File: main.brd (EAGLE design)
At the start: 120 x 120 mm, 578 parts, among them CN1 50 PIN 0.5MM, CN2 10067847-001RLF, CN3 632723300011, CN4 FF0881SA1, CN5 15PIN 0.5MM, CN6 31 PIN FPC, Q1 2N7002, Q2 FDN302P, Q3 2N7002, Q5 SI7489DP, SW2 TACT, SW3 TACT, SW4 TACT, SW5 TACT, SW7 TACT, SW8 SLIDE SPDT, U1 GMAX0505-DV, U10 TPS70950, U11 FT601Q, U12 CBTU02043, U13 MAX25300B, U14 ESP32, U15 MAX25300B, U16 INA180, U17 AP62301, U18 AP62301, U19 SCHMITT, U2 XC7Z014S-1CLG484C, U20 MAX25300B, U21 NOT, U22 MAX25300B, U23 SN74LVC1G3, U24 NAND, U25 EMC1812T, U26 BIPOLAR HALL, U27 LM2663, U28 ADS7867, U29 LM2663, U3 IS43TR16128CL-125KBLI, U30 LM2731X, U31 USBLC6-2SC6, U32 MAX1735, U33 MP2148, U34 TPS22917, U35 AP62301, U36 TLV61046A, U37 W25Q128JV, U38 TPS70918, U39 AP62301, U4 AP63300WU-7, U5 STM32L431RBT, U6 USB ESD, U7 ACT2861QI301-T, U8 TPS70918, U9 STUSB4500

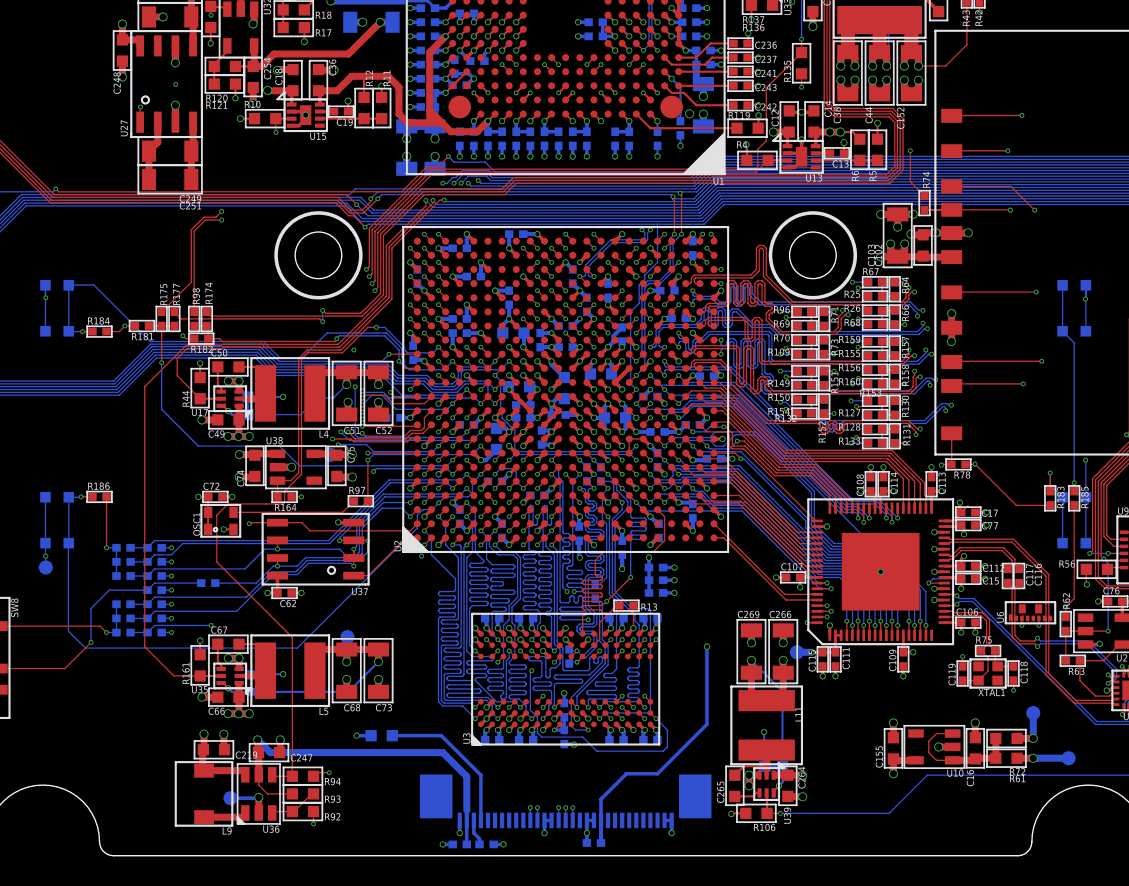
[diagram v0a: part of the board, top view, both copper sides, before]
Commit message: Correct FPGA footprint routed. A lot of work to length match, optimise and review
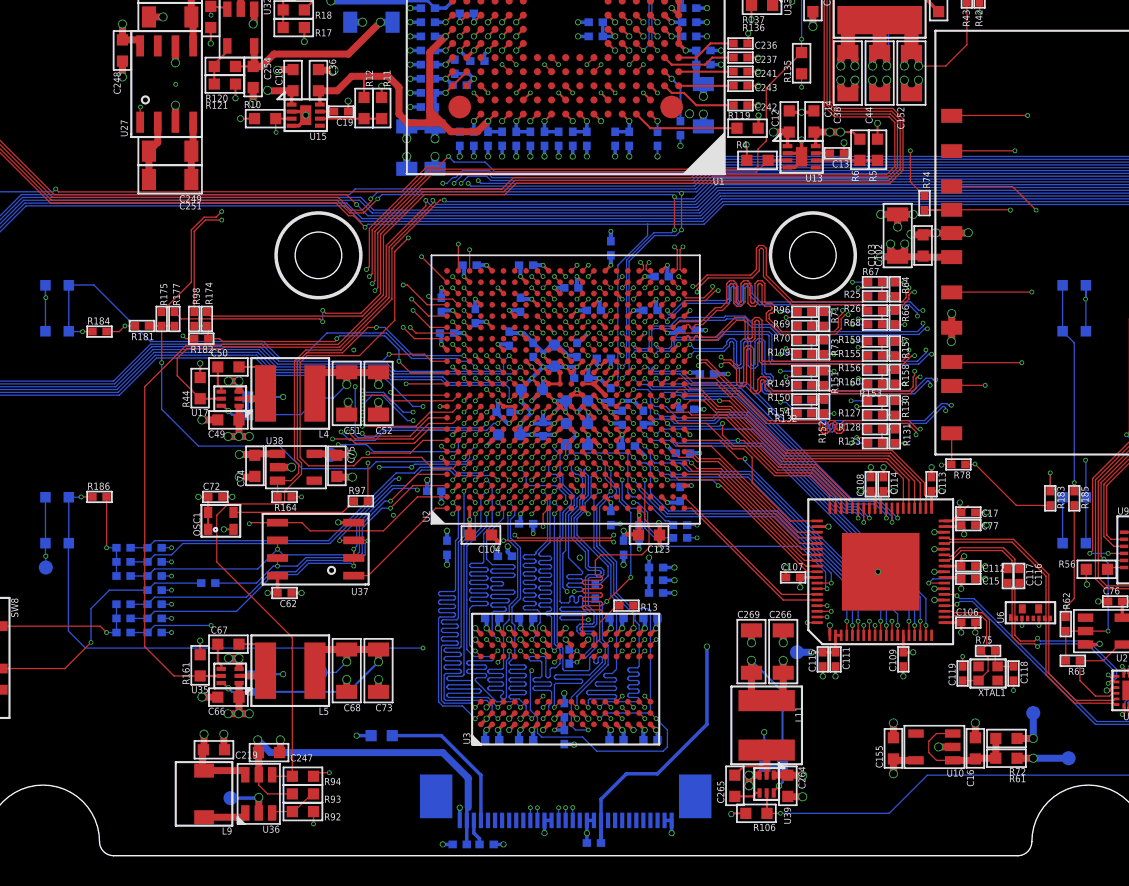
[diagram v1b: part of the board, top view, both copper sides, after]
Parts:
- removed C124, C126: 0.1uF 10V, c_0402:0402
- C104, C123: value 0.1uF 10V -> 47uF 6.3V; device c_0402:0402 -> c_0603:0603
- U2: device ICs:FBGA484 -> ICs:CLG484
- moved C131 17.3 mm to (6.80, -19.0)
- moved C123 16.9 mm to (5.90, -37.3), flipped to the top, turned to 180 degrees
- moved C132 13.9 mm to (0.80, -24.2), turned to 90 degrees
- moved C133 12.1 mm to (0.40, -19.8), turned to 0 degrees
- moved C104 8.83 mm to (-6.00, -37.3), flipped to the top
- moved C127 8.27 mm to (2.00, -21.4), turned to 180 degrees
- moved C138 7.57 mm to (-3.20, -21.0), turned to 270 degrees
- moved R1 7.52 mm to (8.10, -36.6), turned to 0 degrees
- moved R2 7.18 mm to (8.10, -37.5), turned to 180 degrees
- moved C128 6.53 mm to (10.0, -25.9)
- moved C86 5.71 mm to (0.80, -30.9), turned to 180 degrees
- moved C120 4.50 mm to (4.00, -29.0), turned to 90 degrees
- moved C186 4.36 mm to (-9.30, -34.2), turned to 180 degrees
- moved C83 4.21 mm to (-2.40, -27.0), turned to 0 degrees
- moved C122 4.20 mm to (3.20, -27.4), turned to 270 degrees
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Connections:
- removed net N$19: U2.M20
- removed net N$31: U2.M19
- net DDR_D0: now also U2.E1; no longer U2.E3
- net DDR_D2: now also U2.G2; no longer U2.G1
- net DDR_D4: now also U2.L2; no longer U2.L1
- net DDR_D6: now also U2.L1; no longer U2.L2
- net DDR_D8: now also U2.G1; no longer U2.G2
- net DDR_D9: now also U2.E3; no longer U2.E1
- net FT_BE0: now also U2.V4; no longer U2.U4
- net FT_BE1: now also U2.U6; no longer U2.Y5
- net FT_BE3: now also U2.U5; no longer U2.V5
- net FT_D0: now also U2.AA12; no longer U2.AB12
- net FT_D1: now also U2.AB12; no longer U2.AA12
- net FT_D10: now also U2.W10; no longer U2.V10
- net FT_D11: now also U2.AB10; no longer U2.Y10
- net FT_D12: now also U2.Y10; no longer U2.AB10
- net FT_D24: now also U2.U4; no longer U2.V4
- net FT_D29: now also U2.T6; no longer U2.R7
- net FT_D3: now also U2.AA11; no longer U2.AB11
- net FT_D30: now also U2.R7; no longer U2.T6
- net FT_D4: now also U2.AB11; no longer U2.AA11
- net FT_D6: now also U2.V12; no longer U2.U12
- net FT_D7: now also U2.U12; no longer U2.V12
- net FT_GPIO0: now also U2.W8; no longer U2.V8
- net FT_GPIO1: now also U2.V10; no longer U2.W10
- net FT_NRESET: now also U2.V8; no longer U2.Y8
- net FT_NSIWU: now also U2.Y5; no longer U2.U6
- net FT_NTXE: now also U2.V5; no longer U2.U5
- net FT_NWAKEUP: now also U2.Y8; no longer U2.W8
- net GND: no longer C124.1, C126.1
- net PWR_ANA_1V8: no longer C104.2
- net PWR_DDR3_1V35: now also C104.2, C123.2
- net PWR_SEN_0V7_EN: now also U2.A9; no longer U2.B10
- net PWR_SEN_N1V3A_EN: now also U2.B10; no longer U2.A9
- net PWR_SYS_1V8: no longer C123.2, C124.2, C126.2
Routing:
- net BTN_TOPLEFT: track 56.6 -> 108.3 mm
- net BTN_BTMLEFT: track 52.6 -> 103.9 mm, vias 3 -> 2
- net PSS_SD_D0: track 75.0 -> 47.5 mm
- net PSS_SD_D1: track 74.9 -> 48.4 mm
- net PSS_SD_CLK: track 74.7 -> 57.2 mm
- net SEN_B_D12_N: track 35.1 -> 22.5 mm
- net SEN_B_D12_P: track 35.1 -> 22.8 mm
- net N$42: track 1.41 -> 13.1 mm, vias 1 -> 2
- net N$7: track 1.41 -> 12.8 mm
- net PSS_SD_D3: track 74.8 -> 63.9 mm
- net PSS_SD_CMD: track 75.3 -> 65.3 mm
- net PSS_NRST: track 143.9 -> 153.5 mm
- net DDR_A10: track 25.0 -> 15.8 mm
- net PWR_SYS_3V3: track 177.0 -> 168.8 mm
- net BTN_BTMRIGHT: track 43.4 -> 51.3 mm, vias 2 -> 3
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
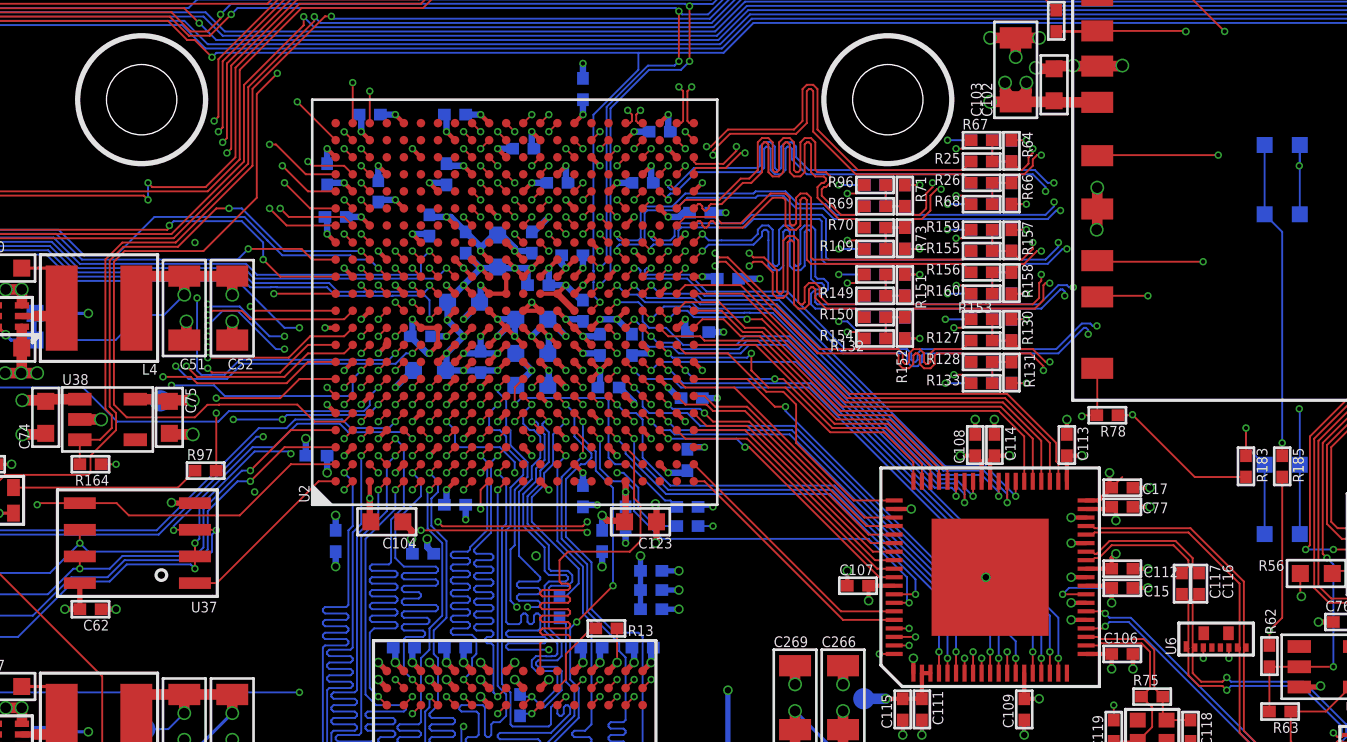
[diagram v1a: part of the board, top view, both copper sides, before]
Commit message: Passes DRC
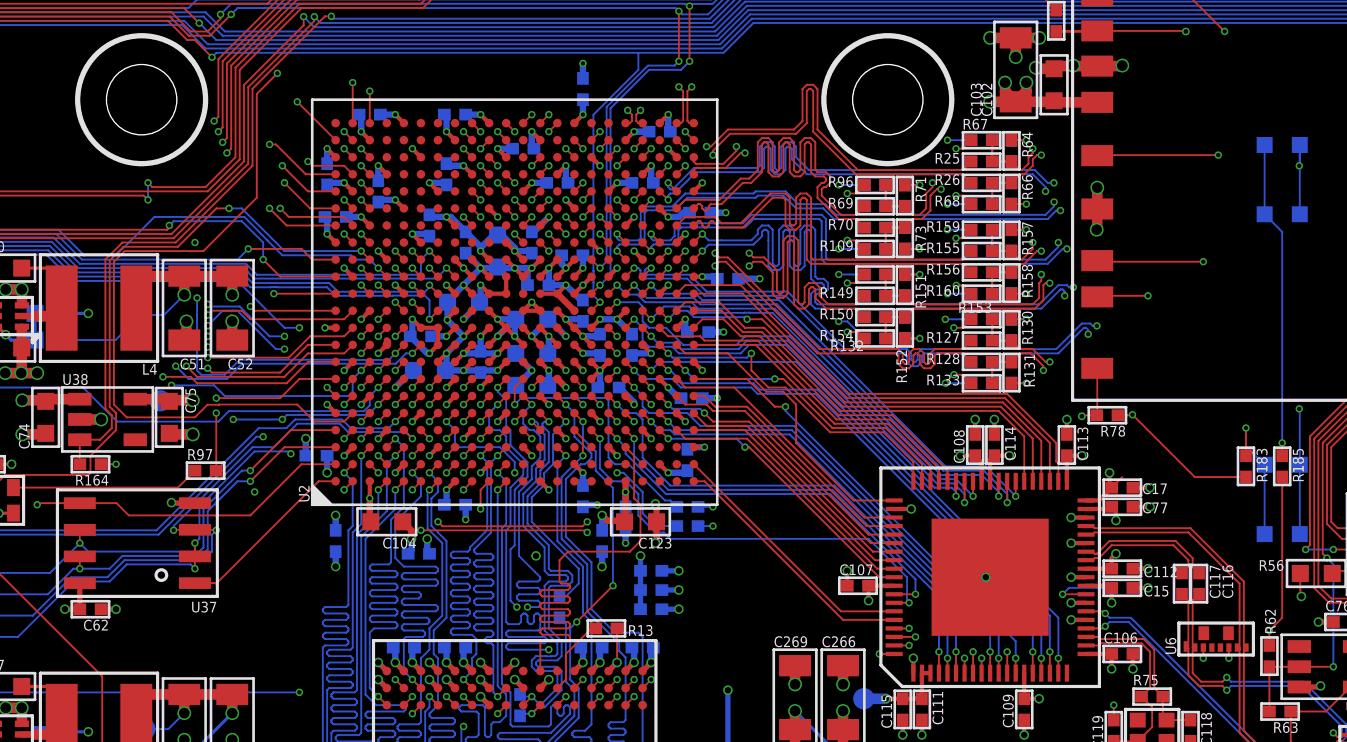
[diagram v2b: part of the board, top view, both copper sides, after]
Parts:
- moved C156 0.20 mm to (-4.50, -38.8)
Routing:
- net PWR_ANA_1V8: track 18.7 -> 19.4 mm

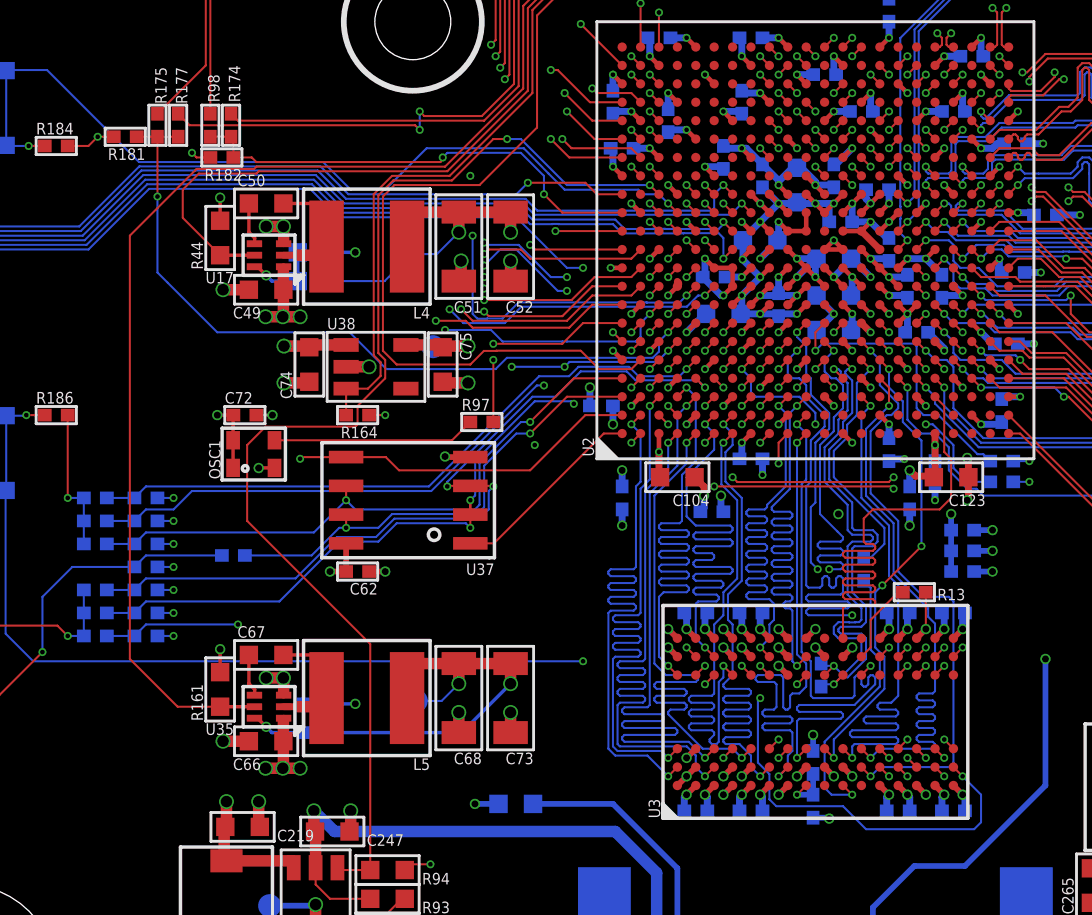
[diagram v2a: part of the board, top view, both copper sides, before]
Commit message: DDR3 length matched
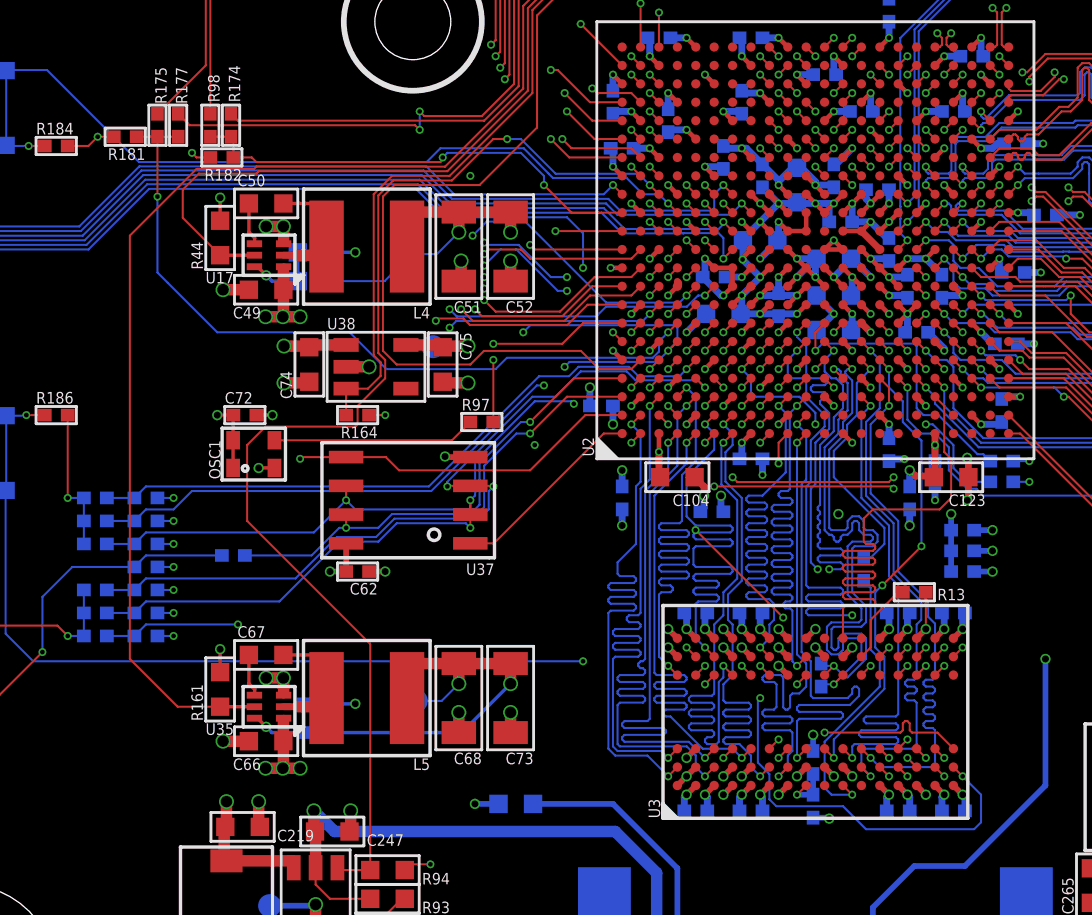
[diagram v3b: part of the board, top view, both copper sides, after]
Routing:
- net DDR_A10: track 15.8 -> 25.0 mm
- net DDR_A3: track 29.6 -> 25.0 mm
- net PSS_SPI_SCLK: track 170.8 -> 175.2 mm
- net DDR_D9: track 29.2 -> 24.9 mm
- net DDR_CLK_P: track 21.2 -> 24.8 mm
- net DDR_CLK_N: track 21.5 -> 24.8 mm
- net DDR_A13: track 28.0 -> 25.1 mm, vias 2 -> 4
- net DDR_D4: track 27.9 -> 25.0 mm
- net DDR_D14: track 27.6 -> 25.0 mm
- net DDR_D1: track 27.3 -> 25.0 mm
- net DDR_DM0: track 27.3 -> 25.0 mm
- net DDR_NCAS: track 27.3 -> 25.1 mm
- net DDR_A9: track 22.8 -> 25.0 mm
- net DDR_A0: track 27.2 -> 25.0 mm
- net DDR_D2: track 27.2 -> 25.0 mm
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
